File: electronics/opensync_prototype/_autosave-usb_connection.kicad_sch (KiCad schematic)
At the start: 4 parts

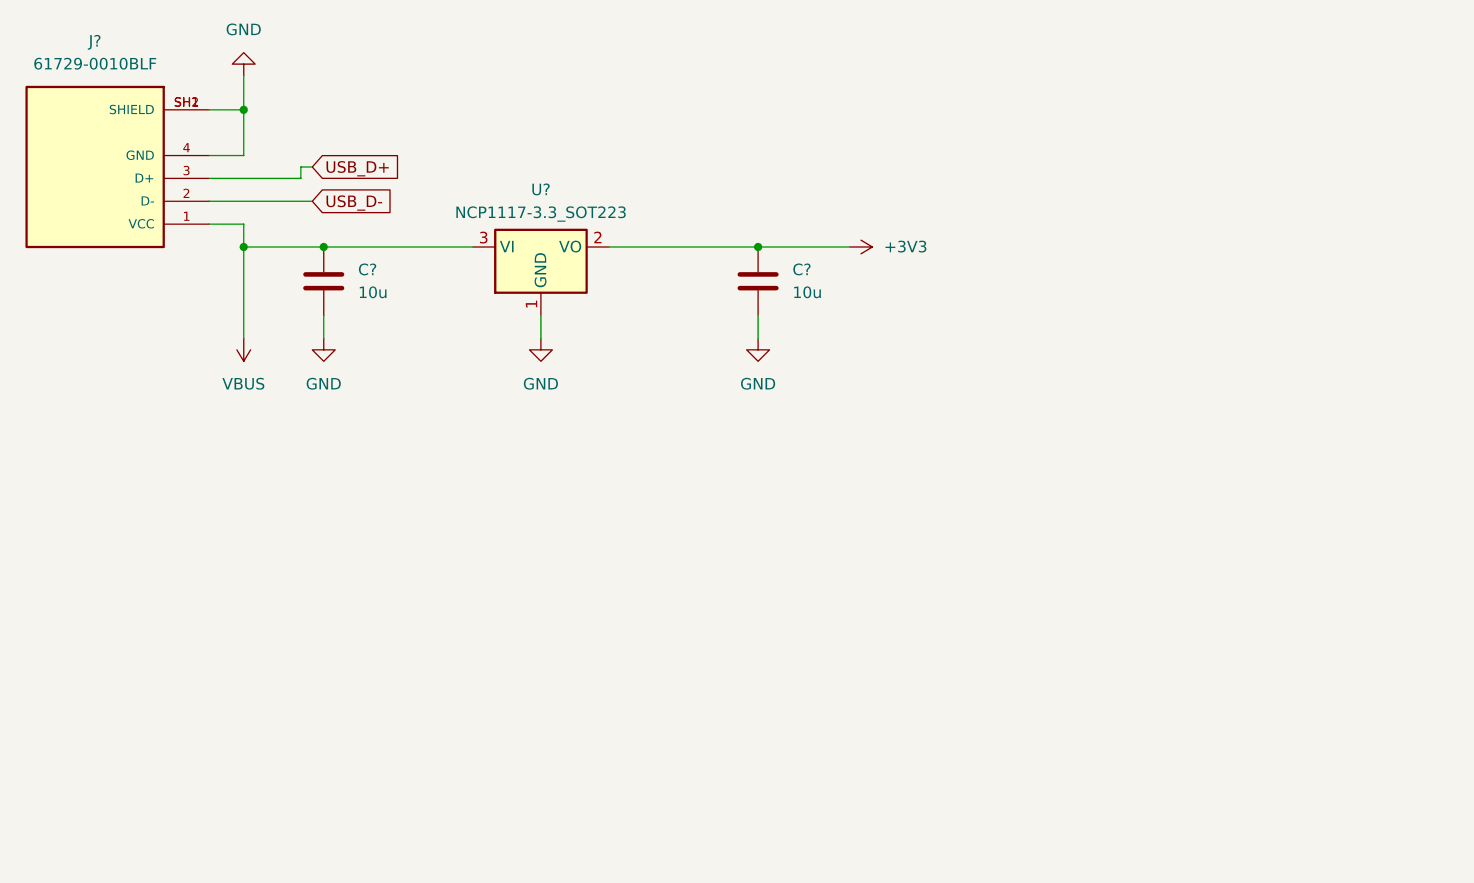
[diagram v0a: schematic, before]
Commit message: KiCAD backup
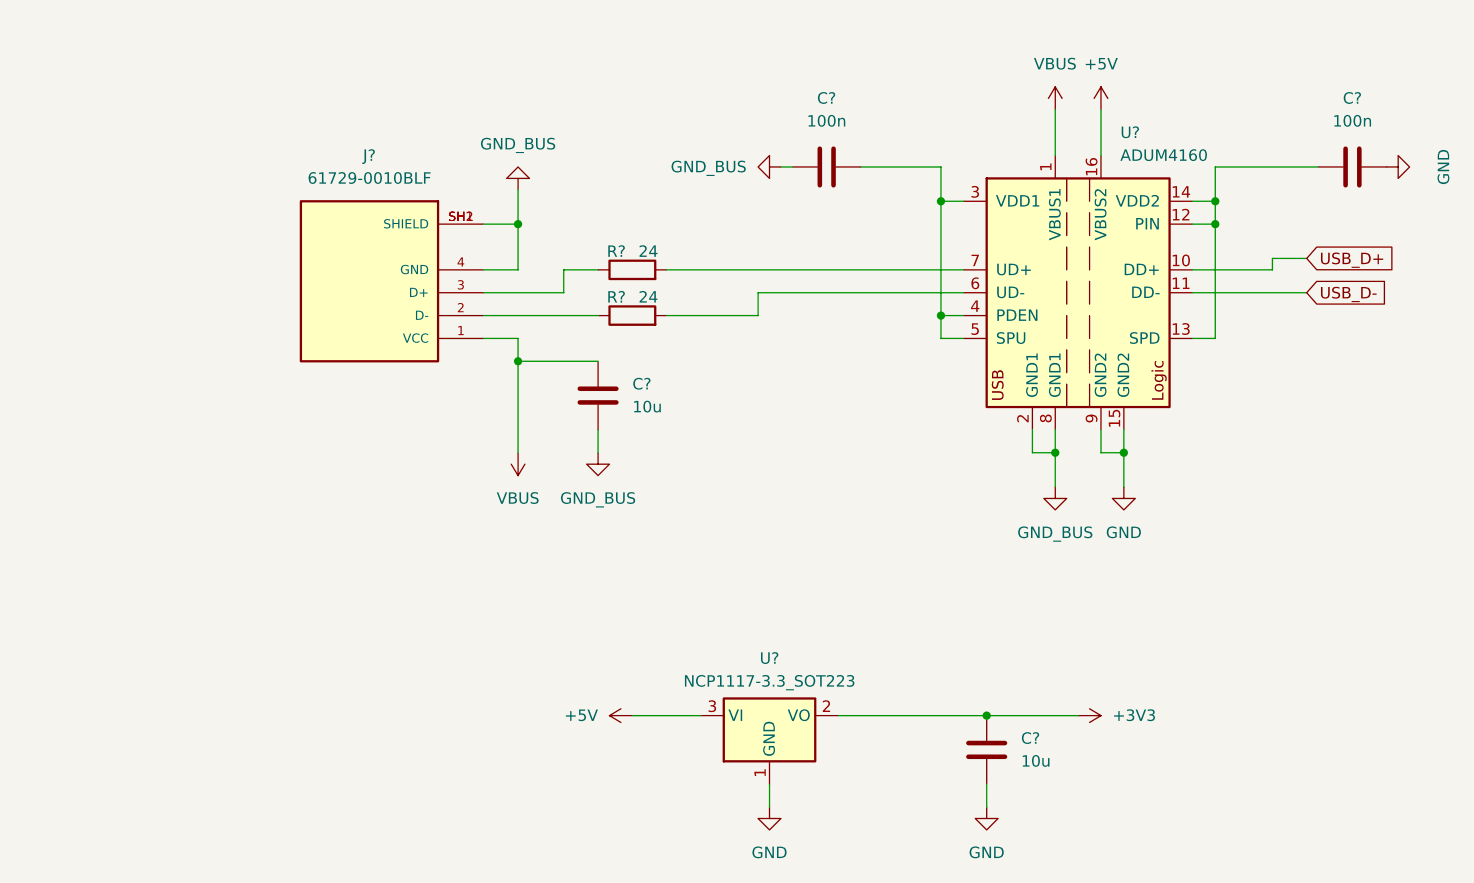
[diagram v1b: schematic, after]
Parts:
- added C? (x2): 100n, symbol Device:C
- added R? (x2): 24, symbol Device:R
- added U?: ADUM4160, Package_SO:SOIC-16W_7.5x10.3mm_P1.27mm, symbol Interface_USB:ADUM4160
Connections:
- net GND: now also C?.2, U?.15 (GND2), U?.9 (GND2); no longer C?.2, J?.4 (GND), J?.SH1 (SHIELD), J?.SH2 (SHIELD)
- net USB_D+: now also U?.10 (DD+); no longer J?.3 (D+)
- net USB_D-: now also U?.11 (DD-); no longer J?.2 (D-)
- net VBUS: now also U?.1 (VBUS1); no longer U?.3 (VI)
- new net: J?.3 (D+), R?.1
- new net: R?.2, U?.7 (UD+)
- new net: J?.2 (D-), R?.1
- new net: C?.1, U?.12 (PIN), U?.13 (SPD), U?.14 (VDD2)
- new net: C?.2, U?.3 (VDD1), U?.4 (PDEN), U?.5 (SPU)
- new net: R?.2, U?.6 (UD-)
- new net +5V: U?.16 (VBUS2), U?.3 (VI)
- new net GND_BUS: C?.1, C?.2, J?.4 (GND), J?.SH1 (SHIELD), J?.SH2 (SHIELD), U?.2 (GND1), U?.8 (GND1)
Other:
- moved on the sheet: C?, J?, U?
